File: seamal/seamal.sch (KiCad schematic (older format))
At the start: 18 parts, among them J1 Conn_01x02_Female, J2 Conn_01x03_Female, J3 Conn_01x02_Female, M1 Motor_DC, SW2 SW_DIP_x02, U1 STM32F303K8Tx, U2 BMX055, U3 DRV8830, U4 W25Q128JVS

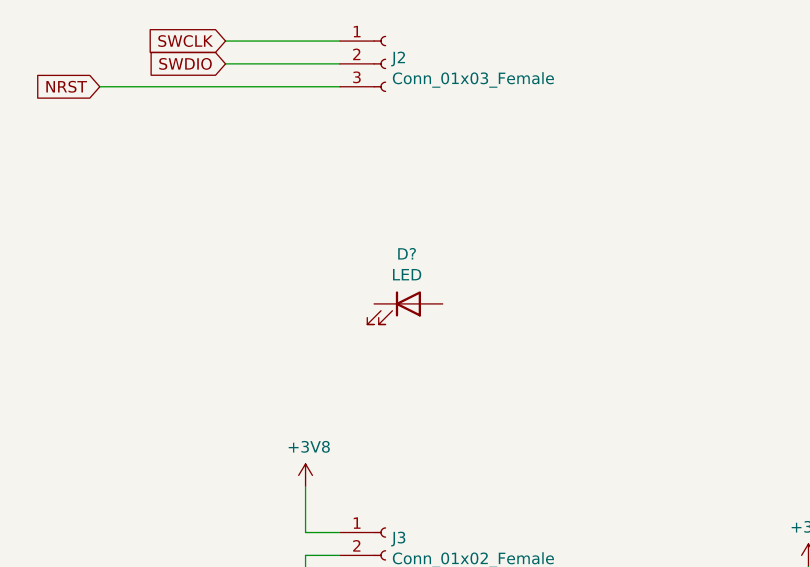
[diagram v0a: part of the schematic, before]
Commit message: deleted
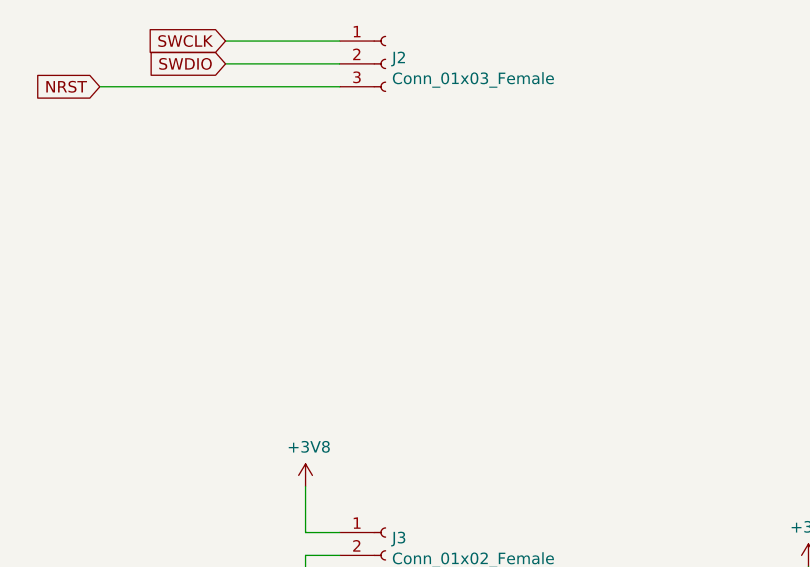
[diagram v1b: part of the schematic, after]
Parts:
- removed D?: LED, symbol Device:LED
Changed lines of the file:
@@
 $EndComp
 NoConn ~ 2250 2500
-$Comp
-L Device:LED D?
-U 1 1 61727B42
-P 6500 2600
-F 0 "D?" H 6493 2817 50  0000 C CNN
-F 1 "LED" H 6493 2726 50  0000 C CNN
-F 2 "" H 6500 2600 50  0001 C CNN
-F 3 "~" H 6500 2600 50  0001 C CNN
-	1    6500 2600
-	1    0    0    -1
-$EndComp
 $EndSCHEMATC

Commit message: commit
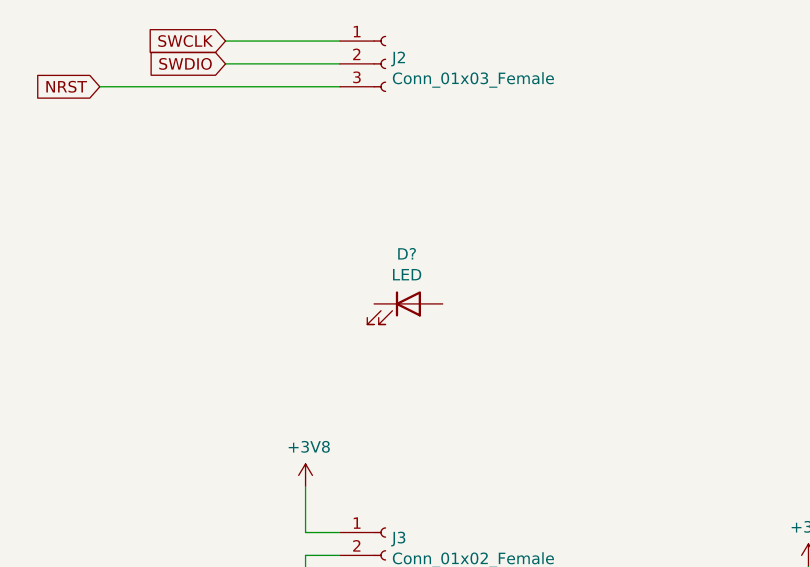
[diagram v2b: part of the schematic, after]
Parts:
- added D?: LED, symbol Device:LED
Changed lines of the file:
@@
 $EndComp
 NoConn ~ 2250 2500
+$Comp
+L Device:LED D?
+U 1 1 61727B42
+P 6500 2600
+F 0 "D?" H 6493 2817 50  0000 C CNN
+F 1 "LED" H 6493 2726 50  0000 C CNN
+F 2 "" H 6500 2600 50  0001 C CNN
+F 3 "~" H 6500 2600 50  0001 C CNN
+	1    6500 2600
+	1    0    0    -1
+$EndComp
 $EndSCHEMATC
